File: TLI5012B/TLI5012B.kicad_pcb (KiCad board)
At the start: 2 copper layers, 13.2 x 13.2 mm, 7 parts, among them J1 Conn_01x05_Female, U1 TLI5012B

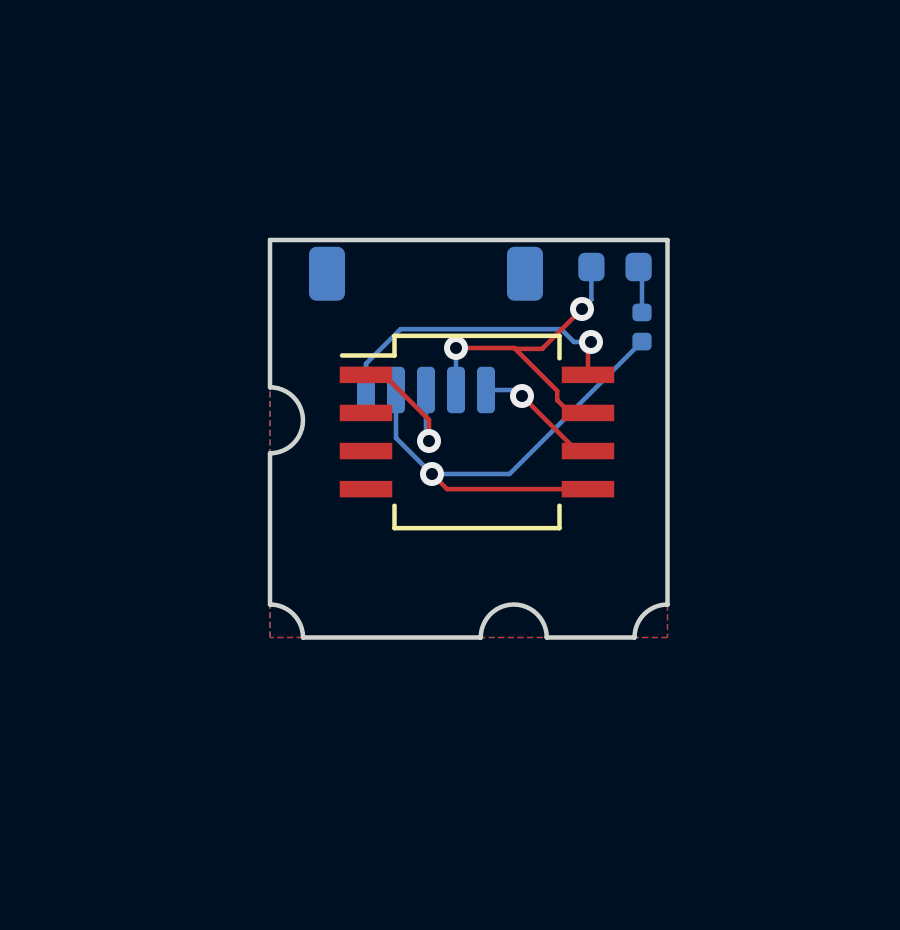
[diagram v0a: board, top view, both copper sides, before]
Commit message: with pcb for walkera_wk-ws-028-014A
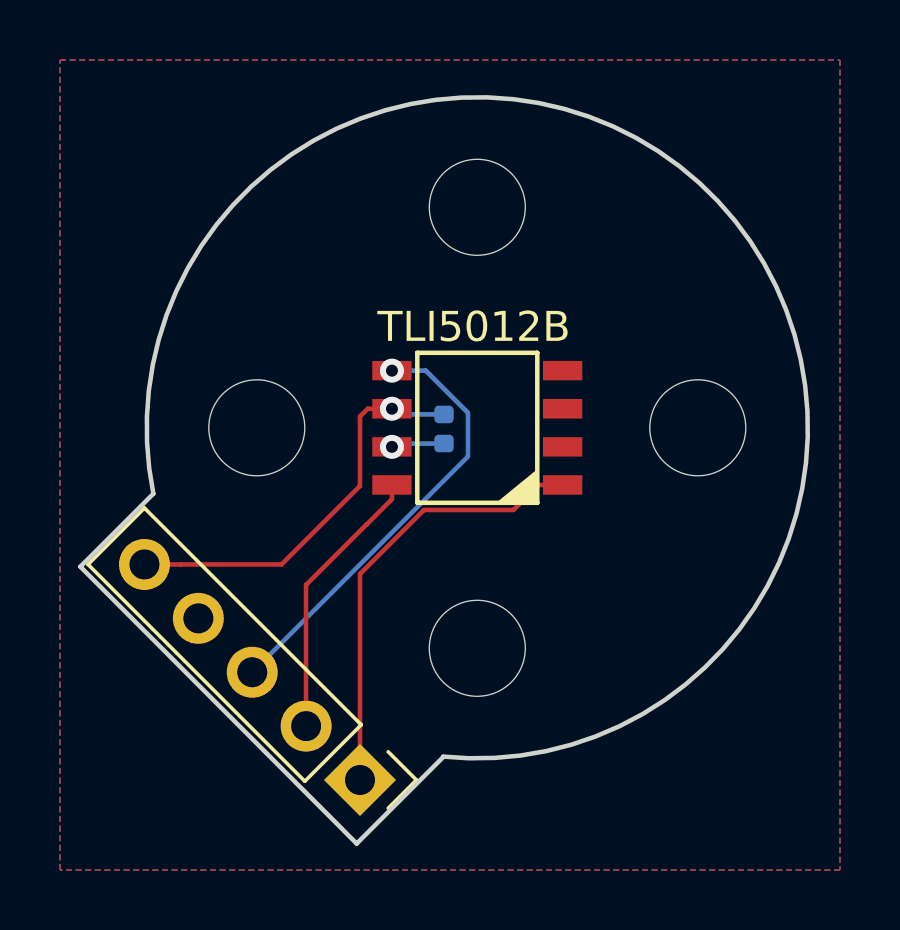
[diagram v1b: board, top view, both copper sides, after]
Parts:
- removed D1: LED, LED_SMD:LED_0603_1608Metric
- removed G***: LOGO, custom_lib:R1_eyes_mask_5.5mm
- removed G***: LOGO, custom_lib:R1_face_mask_5.5mm
- removed G***: LOGO, custom_lib:R1_ear_silk_5.5mm
- removed R1: 1k, LED_SMD:LED_0402_1005Metric
- added C1: C, Capacitor_SMD:C_0402_1005Metric, B.Cu at (136.7, 86.4)
- added H1: MountingHole, MountingHole:MountingHole_3.2mm_M3, F.Cu at (137.8, 93.7)
- added H2: MountingHole, MountingHole:MountingHole_3.2mm_M3, F.Cu at (137.8, 79.0)
- added H3: MountingHole, MountingHole:MountingHole_3.2mm_M3, F.Cu at (130.4, 86.4)
- added H4: MountingHole, MountingHole:MountingHole_3.2mm_M3, F.Cu at (145.1, 86.4)
- J1: footprint Connector_JST:JST_SH_SM05B-SRSS-TB_1x05-1MP_P1.00mm_Horizontal -> Connector_PinHeader_2.54mm:PinHeader_1x05_P2.54mm_Vertical; moved to F.Cu
- U1: footprint Package_SO:SO-8_5.3x6.2mm_P1.27mm -> custom_lib:TLI5012B
- moved J1 15.2 mm to (133.9, 98.1), turned to 225 degrees
- moved U1 0.14 mm to (137.8, 86.4), turned to 90 degrees
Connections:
- J1 pad 1: /IFB -> /IFC
- J1 pad 2: /IFA -> /IFB
- J1 pad 3: /IFC -> /IFA
- J1 pad 4: /GND -> GND
- J1 pad 5: /VDD -> +5V
- U1 pad 6: /VDD -> +5V
- U1 pad 7: /GND -> GND
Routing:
- net +5V: track 0.00 -> 13.6 mm, vias 0 -> 1
- net /GND: track 11.2 -> 0.00 mm, vias 2 -> 0
- net /IFC: track 5.17 -> 14.9 mm, vias 1 -> 0
- net /VDD: track 4.24 -> 0.00 mm, vias 1 -> 0
- net /IFA: track 17.5 -> 14.7 mm
- net GND: track 0.00 -> 1.78 mm, vias 0 -> 1
- net Net-(D1-Pad2): track 1.56 -> 0.00 mm
- net /IFB: track 10.2 -> 9.23 mm, vias 1 -> 0
- added copper zone on F.Cu, net GND
- removed copper zone on F.Cu, net +5V
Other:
- board size 13.2 x 13.2 mm -> 24.2 x 24.9 mm
- board text added: "100n"
- board text added: "5V"
- board text added: "A"
- board text added: "B"
- board text added: "GND"
- board text added: "I"
- board text added: "TLI5012B"
